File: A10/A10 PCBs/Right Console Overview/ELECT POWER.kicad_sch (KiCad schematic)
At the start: 13 parts, among them J22 ELEC POWER, SW23 L GEN, SW24 APU GEN PWR, SW25 R GEN, SW26 INVTR STBY, SW27 APU GEN PWR, SW28 BATTERY PWR

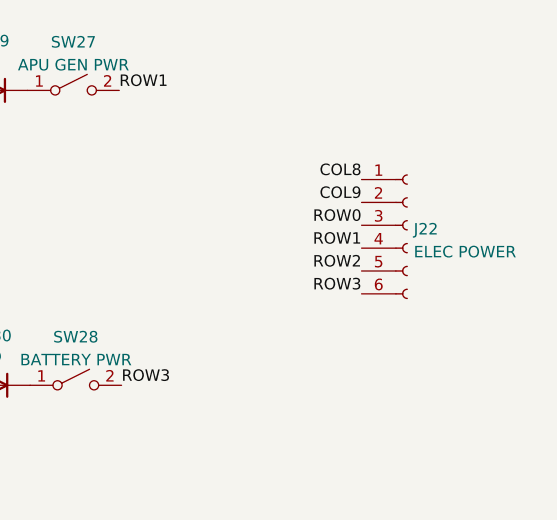
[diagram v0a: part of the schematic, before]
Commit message: a10
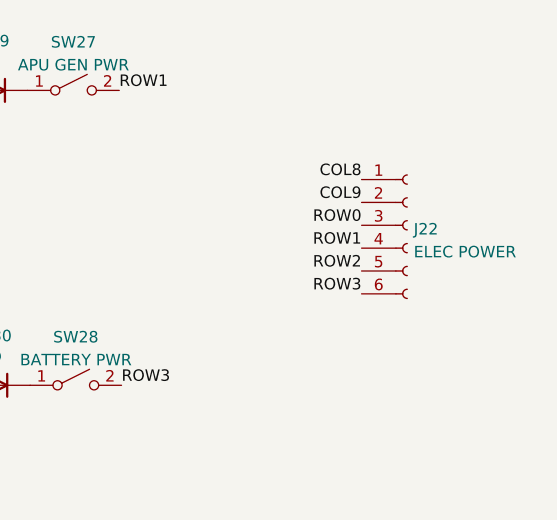
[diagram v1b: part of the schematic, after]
